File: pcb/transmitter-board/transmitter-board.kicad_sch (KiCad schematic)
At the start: 26 parts, among them J1 USB-C_USB-310F-B-SU, Q3 AO3400A, Q4 AO3400A, SW1 SW_DPDT_x2, U1 NE555D, U3 TP4056-42-ESOP8, U4 DW01A

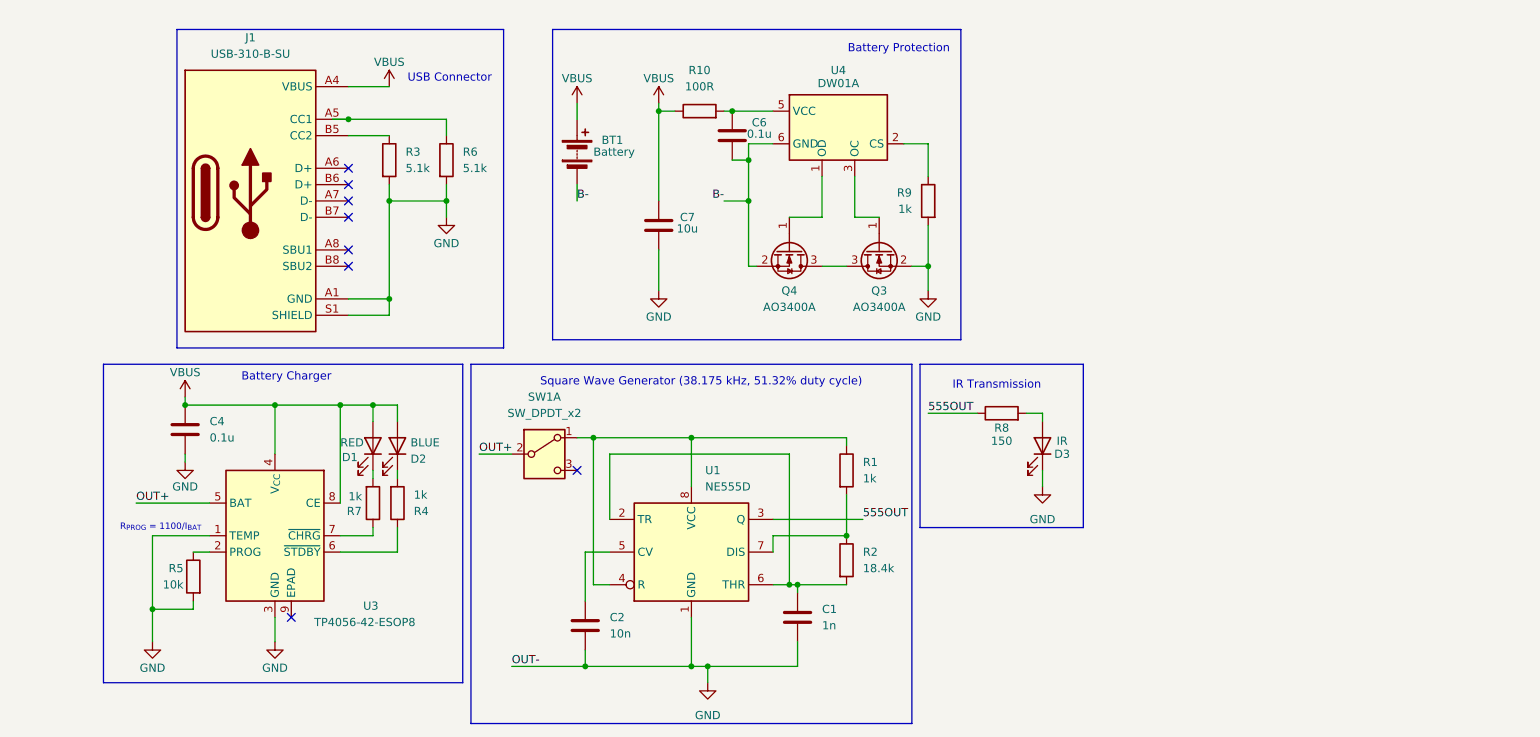
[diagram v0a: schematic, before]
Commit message: Refactor transmitter-board schematic
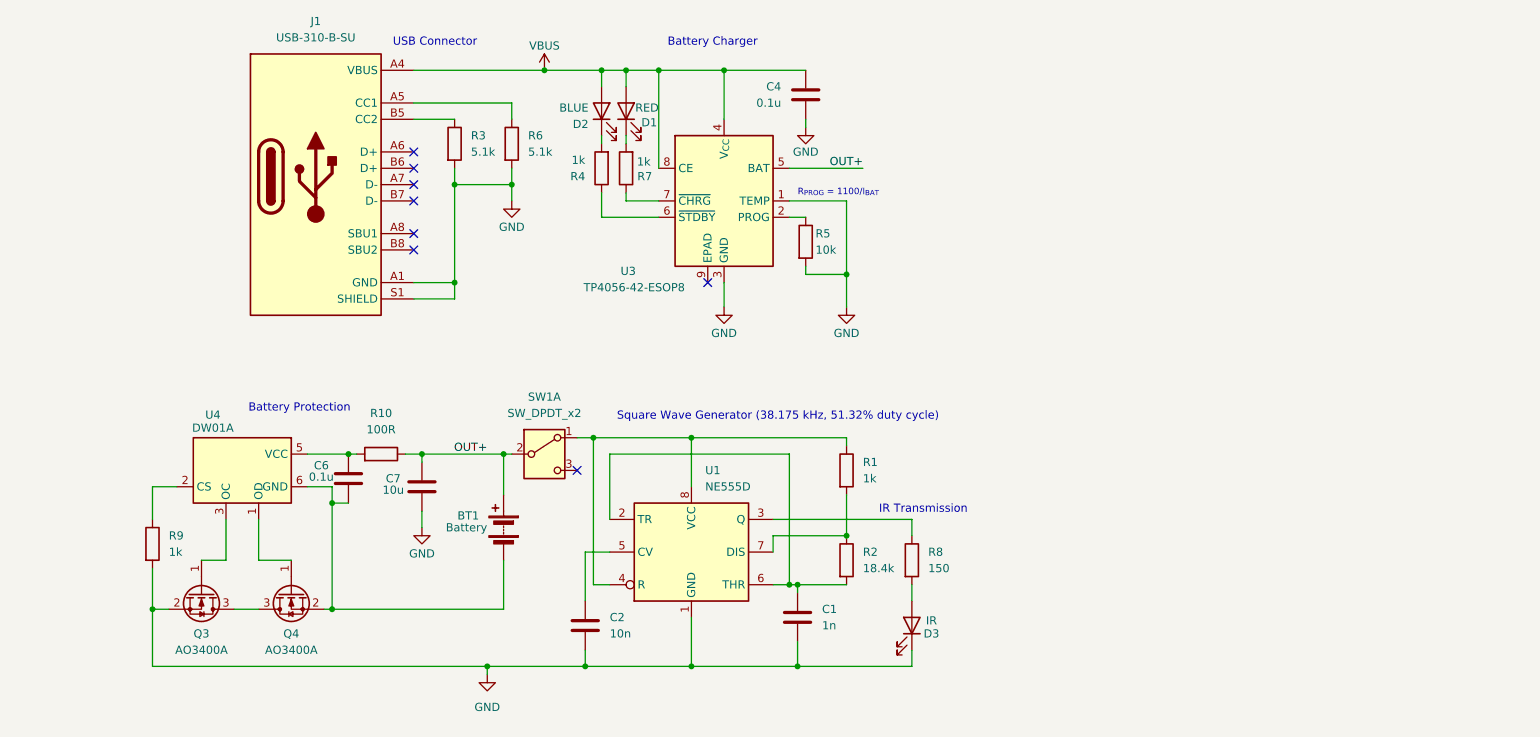
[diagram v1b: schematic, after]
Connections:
- net OUT+: now also BT1.1 (+), C7.1, R10.1
- net VBUS: no longer BT1.1 (+), C7.1, R10.1
- net 555OUT: no longer names the net of R8.1, U1.3 (Q)
- net B-: no longer names the net of BT1.2 (-), C6.2, Q4.2 (S), U4.6 (GND)
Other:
- moved on the sheet: BT1, C4, C6, C7, D1, D2, D3, J1, Q3, Q4, R10, R3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

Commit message: Final refactor transmitter-board schematic
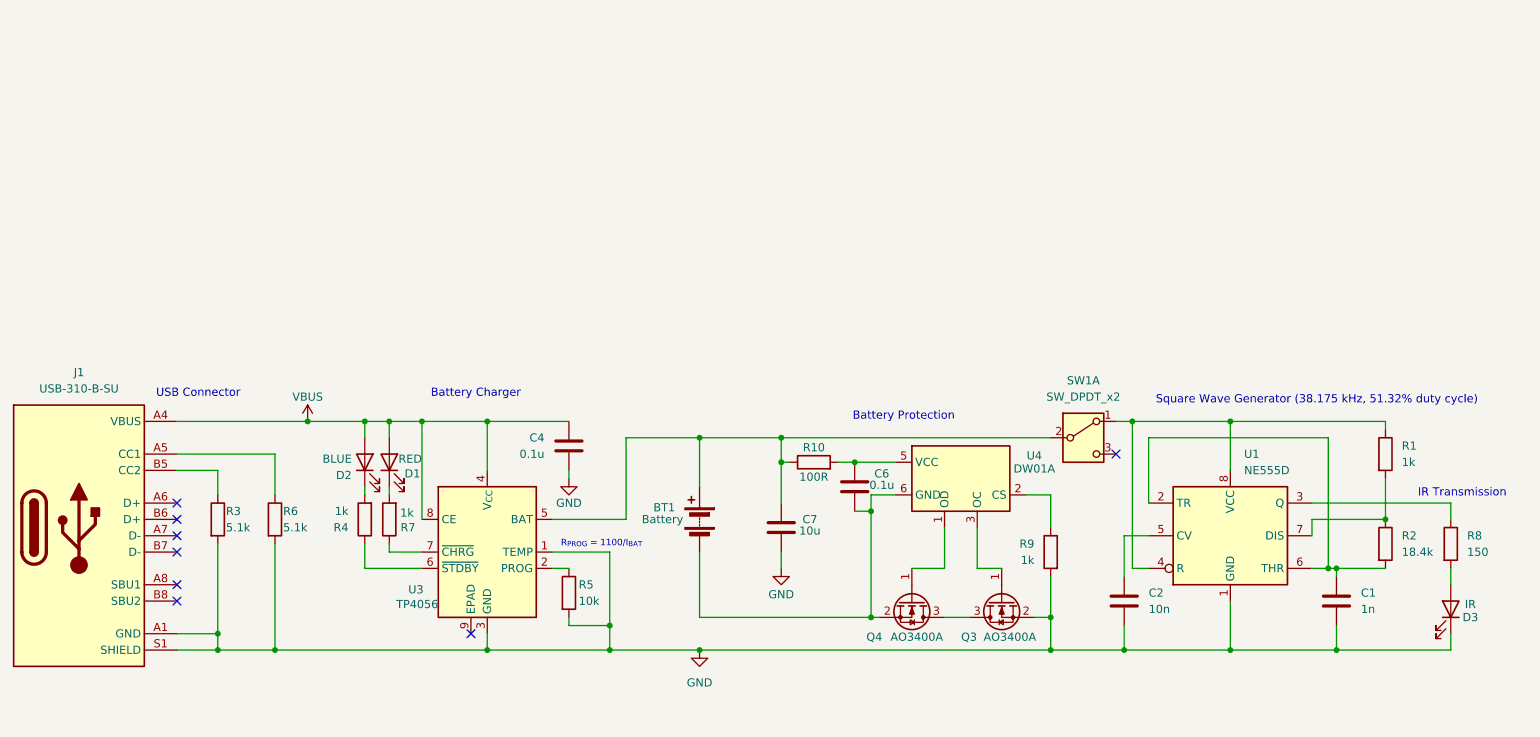
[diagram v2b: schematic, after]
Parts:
- U3: value TP4056-42-ESOP8 -> TP4056
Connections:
- net OUT+: no longer names the net of BT1.1 (+), C7.1, R10.1, SW1.2 (B), U3.5 (BAT)
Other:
- moved on the sheet: BT1, C1, C2, C4, C6, C7, D1, D2, D3, J1, Q3, Q4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
